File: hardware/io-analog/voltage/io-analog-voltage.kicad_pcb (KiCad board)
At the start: 2 copper layers, 60 x 60 mm, 28 parts, among them J1 Analog Extension, J2 Output, J3 Power, J4 Power, U1 TLV2772, U2 TLV2772, U3 LM317T

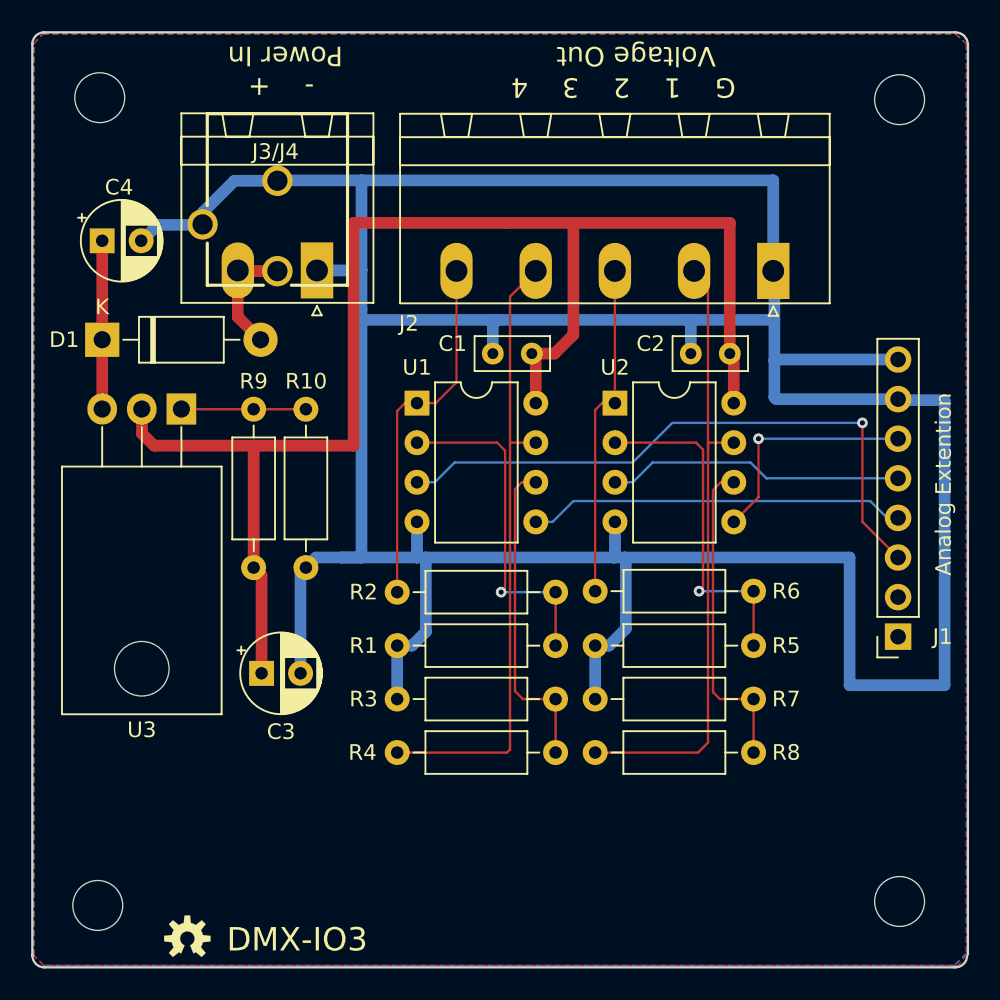
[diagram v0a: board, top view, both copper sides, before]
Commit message: Finalize io-analog boards.
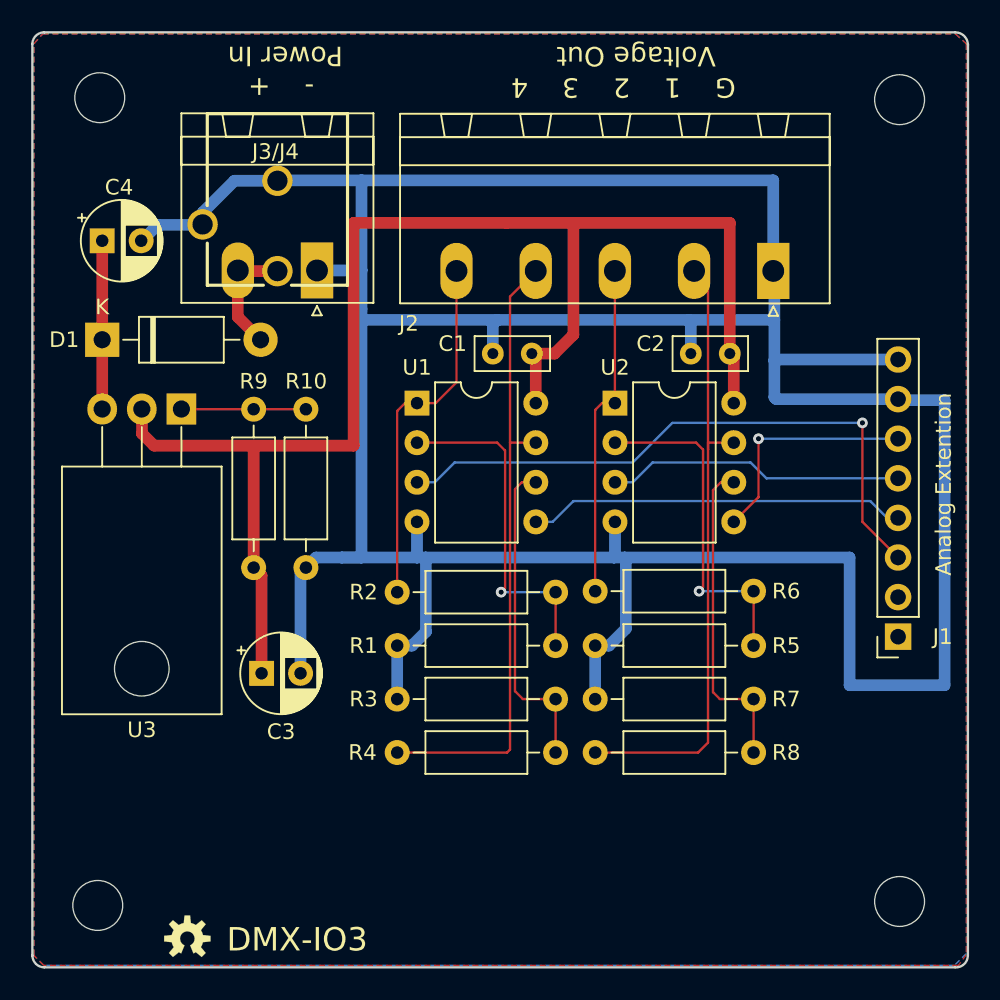
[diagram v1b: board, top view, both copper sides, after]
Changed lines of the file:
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@@
     (pcbplotparams
       (layerselection 0x010fc_ffffffff)
-      (usegerberextensions false)
+      (usegerberextensions true)
       (usegerberattributes false)
       (usegerberadvancedattributes false)
@@
       (psa4output false)
       (plotreference true)
-      (plotvalue true)
+      (plotvalue false)
       (plotinvisibletext false)
       (padsonsilk false)
-      (subtractmaskfromsilk false)
+      (subtractmaskfromsilk true)
       (outputformat 1)
       (mirror false)
-      (drillshape 1)
+      (drillshape 0)
       (scaleselection 1)
-      (outputdirectory ""))
+      (outputdirectory "grb"))
   )
   (net 0 "")
@@
       (xy -1.404739 2.654895) (xy -1.386268 2.656083) (xy -1.36631 2.655905)) (layer B.SilkS) (width 0.01))
   )
+  (gr_arc (start 185.57748 133.0325) (end 185.53178 133.7945) (angle -90) (layer Edge.Cuts) (width 0.15))
   (gr_line (start 411.226 134.8105) (end 411.1625 134.874) (layer Dwgs.User) (width 0.15))
   (gr_text "Analog Extention" (at 184.785 102.8065 90) (layer F.SilkS)
@@
   )
   (gr_line (start 127.0914 73.8175) (end 185.5114 73.8175) (layer Edge.Cuts) (width 0.15))
-  (gr_line (start 186.3472 74.6355) (end 186.342 132.969) (layer Edge.Cuts) (width 0.15))
-  (gr_arc (start 185.5292 133.0325) (end 185.4835 133.7945) (angle -90) (layer Edge.Cuts) (width 0.15))
+  (gr_line (start 186.3472 74.5795) (end 186.342 133.0555) (layer Edge.Cuts) (width 0.15))
   (gr_arc (start 185.5292 74.6355) (end 186.3472 74.6355) (angle -90) (layer Edge.Cuts) (width 0.15))
   (gr_arc (start 127.0914 74.5795) (end 127.0914 73.8175) (angle -90) (layer Edge.Cuts) (width 0.15))
   (gr_arc (start 127.0965 133.0325) (end 126.3345 133.0325) (angle -90) (layer Edge.Cuts) (width 0.15))
-  (gr_line (start 127.0965 133.7945) (end 185.4835 133.7945) (layer Edge.Cuts) (width 0.15))
+  (gr_line (start 127.0914 133.7945) (end 185.5114 133.7945) (layer Edge.Cuts) (width 0.15))
   (gr_line (start 126.3294 133.0555) (end 126.3294 74.5795) (layer Edge.Cuts) (width 0.15))
   (gr_text "DMX-IO3, Rev 1.2\nCrazy Giraffe Software\n\n" (at 147.6375 129.9845) (layer B.SilkS)
